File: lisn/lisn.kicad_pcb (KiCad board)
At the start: 2 copper layers, 50 x 49 mm, 33 parts, among them J1 IN+, J2 IN-, J3 GND, J4 GND, J5 OUT+, J6 OUT-, J7 SMA, SW1 DPDT, T1 SWB2010

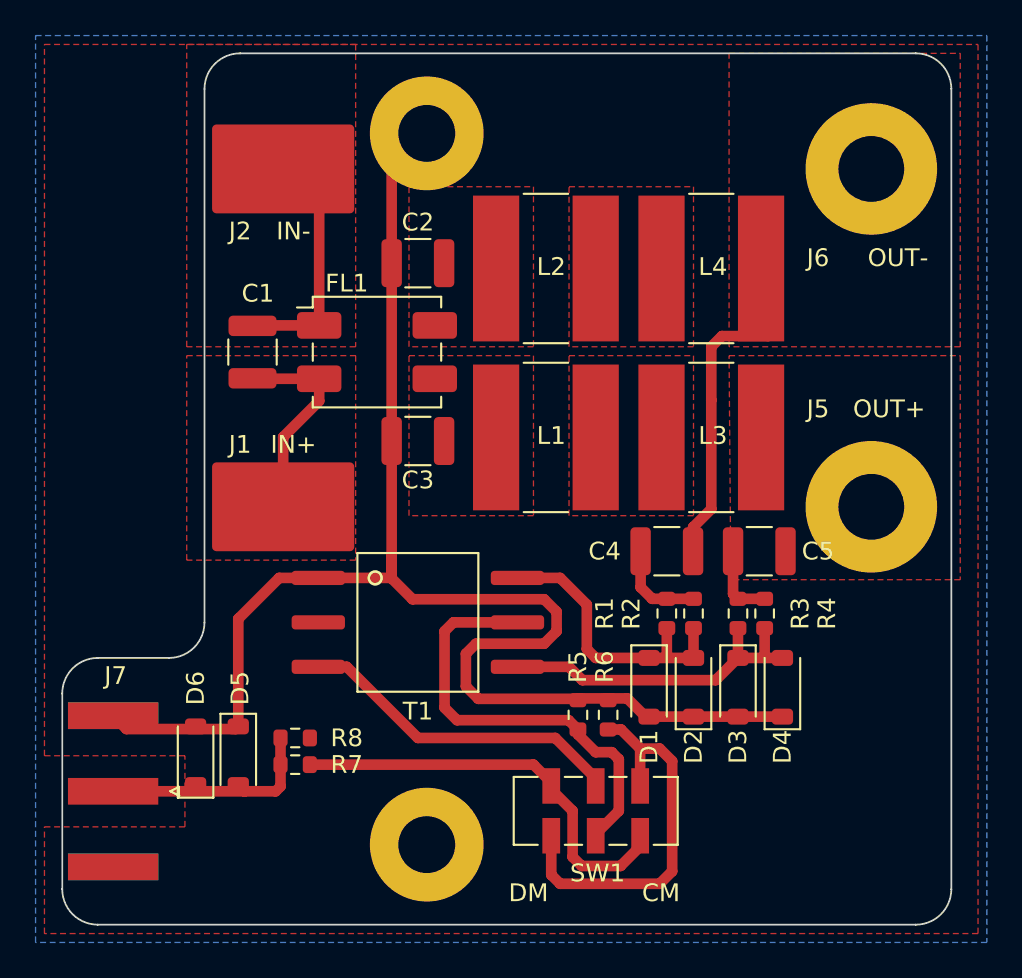
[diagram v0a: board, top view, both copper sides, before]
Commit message: Update LISN PCB
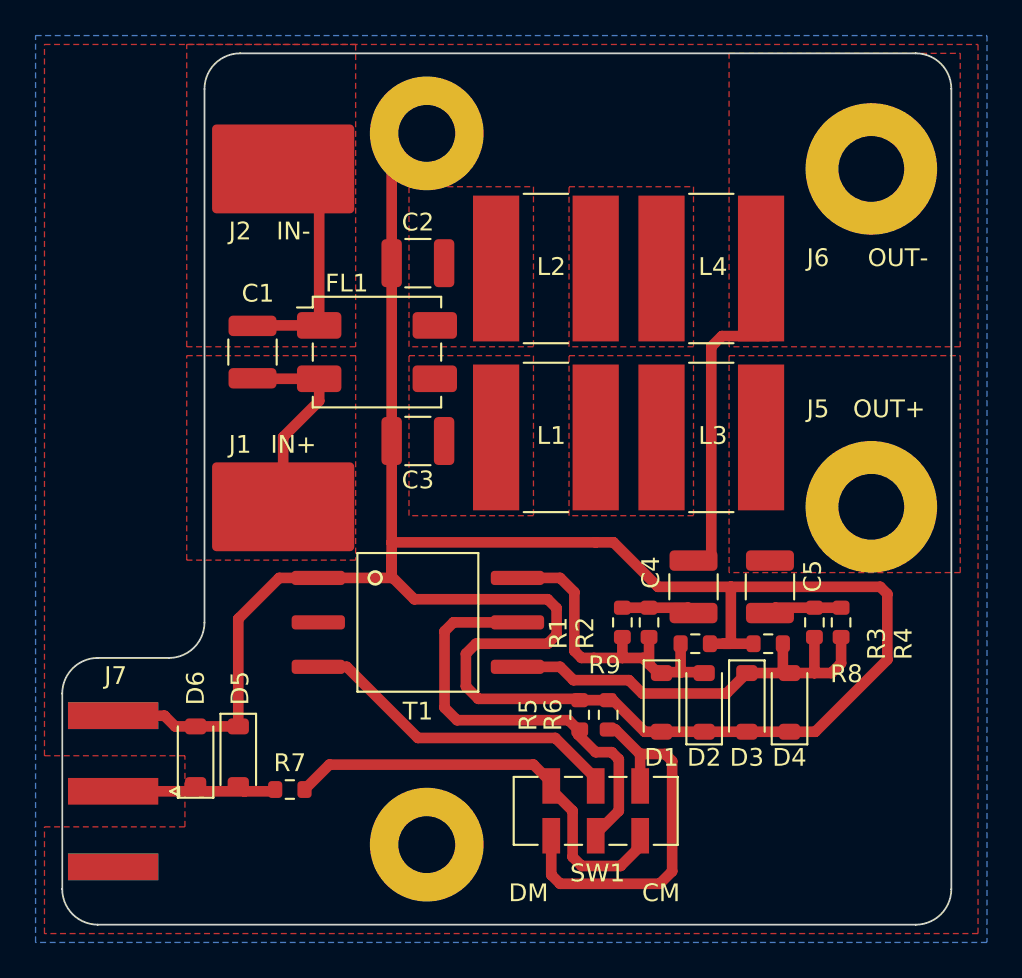
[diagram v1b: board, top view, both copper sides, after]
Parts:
- added R9: 68, Resistor_SMD:R_0603_1608Metric, F.Cu at (160.6, 99.2)
- R5, R6: value 50 -> 82
- R7: value 18 -> 30
- R8: value 82 -> 68
- moved R8 27.1 mm to (164.7, 99.2)
- moved R3 4.33 mm to (167.3, 98.0)
- moved R4 4.33 mm to (168.8, 98.0)
- moved R1 2.55 mm to (156.5, 98.0)
- moved R2 2.55 mm to (158.0, 98.0)
- moved C4 2.50 mm to (160.5, 96.0), turned to -90 degrees
- moved C5 2.09 mm to (164.8, 96.0), turned to -90 degrees
- moved R7 1.43 mm to (137.8, 107.4)
- moved D1 1.10 mm to (158.7, 102.5)
- moved D2 1.04 mm to (161.1, 102.5)
- moved D3 0.99 mm to (163.5, 102.5)
- moved D4 0.94 mm to (165.9, 102.5)
- moved R5 0.10 mm to (154.1, 103.2)
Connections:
- R8 pad 1: GND -> Net-(D3-K)
- R8 pad 2: Net-(D5-A) -> GND
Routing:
- net GND: track 87.4 -> 134.3 mm
- net Net-(D3-K): track 18.9 -> 24.8 mm
- net Net-(D5-A): track 13.4 -> 10.3 mm
- net Net-(D1-K): track 16.4 -> 18.8 mm
- net Net-(C4-Pad2): track 5.27 -> 4.12 mm
- net /OUT_M: track 16.5 -> 17.6 mm
- net /OUTPUT: track 23.7 -> 24.6 mm
